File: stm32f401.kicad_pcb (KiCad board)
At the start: 2 copper layers, 35 x 35 mm, 37 parts, among them J1 USB_C_Receptacle_USB2.0_16P, SW1 SW_Push, SW2 SW_Push, U1 STM32F401RBT6, U2 BMI160, U3 AMS1117-3.3, Y1 16M

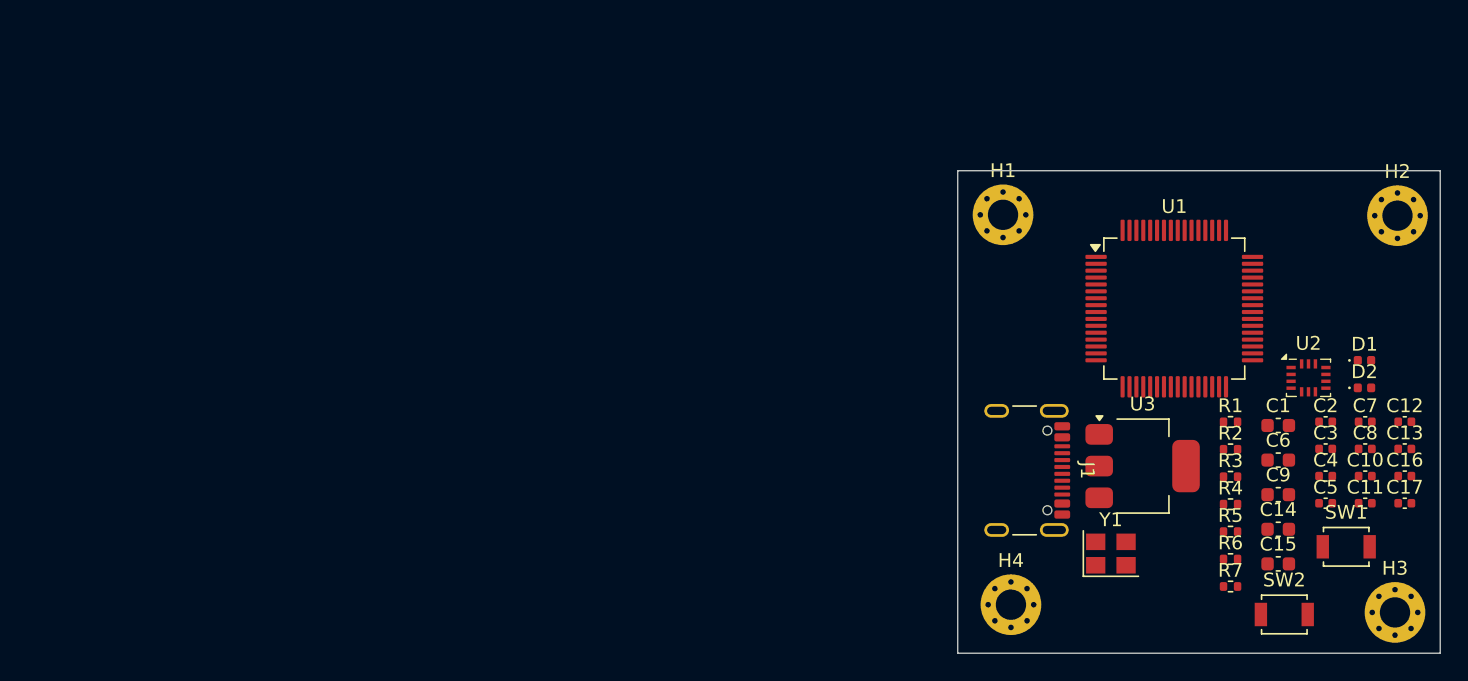
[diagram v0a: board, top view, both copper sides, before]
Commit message: Initial PCB Design
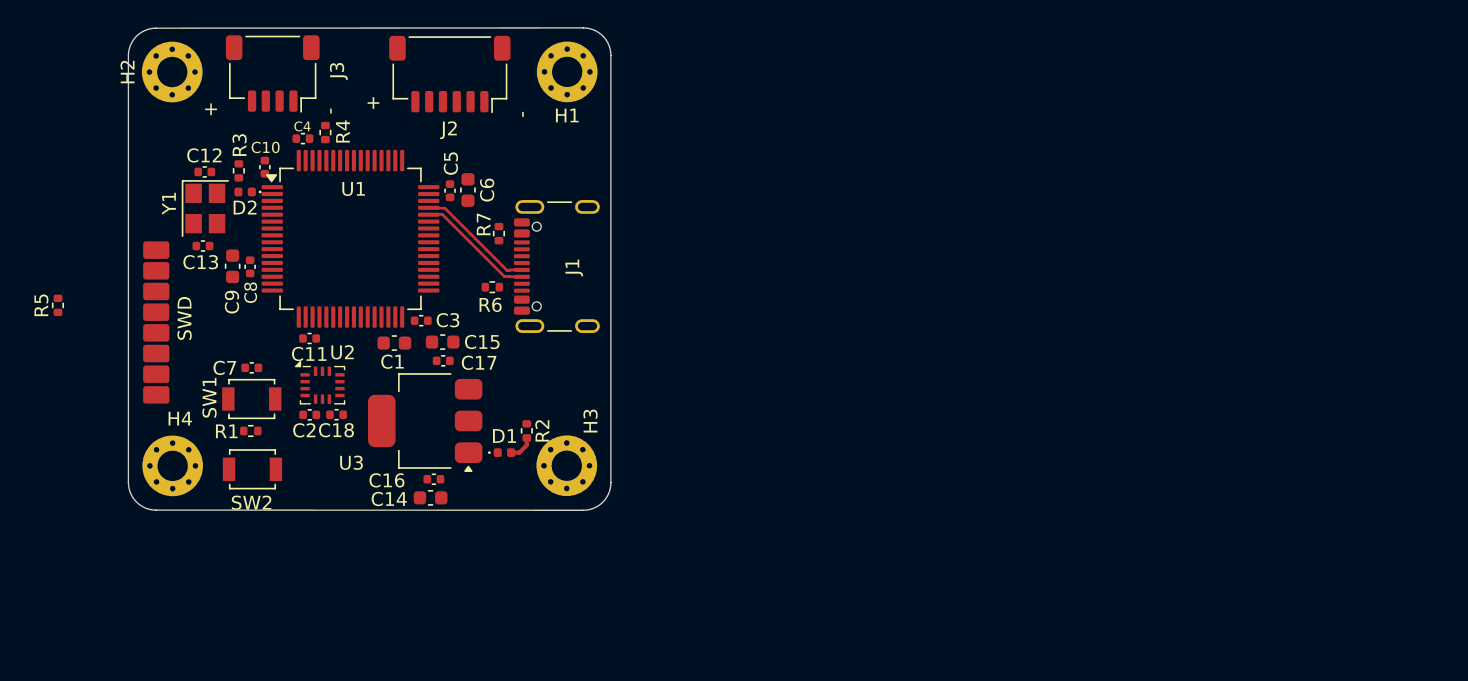
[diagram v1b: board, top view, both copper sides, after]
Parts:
- added C18: .1uF, Capacitor_SMD:C_0402_1005Metric, F.Cu at (55.1, 78.0)
- added J2: Conn_01x06_Pin, Connector_JST:JST_SH_SM06B-SRSS-TB_1x06-1MP_P1.00mm_Horizontal, F.Cu at (63.3, 53.3)
- added J3: Conn_01x04_Pin, Connector_JST:JST_SH_SM04B-SRSS-TB_1x04-1MP_P1.00mm_Horizontal, F.Cu at (50.5, 53.3)
- added SWD: Conn_01x08_Pin, Custom:Conn_0x08, F.Cu at (42.0, 80.6)
- D1: value RED -> R
- D2: value GREEN -> G
- moved H2 89.5 mm to (43.2, 53.2), turned to 90 degrees
- moved C12 88.9 mm to (45.5, 60.4)
- moved C13 88.4 mm to (45.4, 65.8)
- moved R5 86.6 mm to (34.9, 70.1), turned to 90 degrees
- moved C10 82.9 mm to (49.9, 60.1), turned to -90 degrees
- moved D2 82.4 mm to (48.5, 61.9), turned to 180 degrees
- moved C8 82.0 mm to (48.8, 67.3), turned to -90 degrees
- moved C7 80.9 mm to (49.0, 74.6)
- moved SW1 80.1 mm to (49.0, 76.9)
- moved C4 78.1 mm to (52.7, 58.0)
- moved C9 77.6 mm to (47.6, 67.3), turned to -90 degrees
- moved C11 77.5 mm to (53.1, 72.5), turned to 180 degrees
- moved SW2 75.6 mm to (49.0, 82.0)
- moved R3 75.3 mm to (48.0, 60.4), turned to -90 degrees
- moved C2 73.7 mm to (53.1, 78.0)
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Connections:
- net /NRST renamed NRST
- J1 pad S1: unconnected-(J1-SHIELD-PadS1) -> GND
- U1 pad 11: unconnected-(U1-PC3-Pad11) -> T3C4
- U1 pad 16: unconnected-(U1-PA2-Pad16) -> UART2_TX
- U1 pad 17: unconnected-(U1-PA3-Pad17) -> UART2_RX
- U1 pad 2: unconnected-(U1-PC13-Pad2) -> /USR_LED
- U1 pad 20: unconnected-(U1-PA4-Pad20) -> CS
- U1 pad 21: /USR_LED -> SCLK
- U1 pad 22: unconnected-(U1-PA6-Pad22) -> MISO
- U1 pad 23: unconnected-(U1-PA7-Pad23) -> MOSI
- U1 pad 24: unconnected-(U1-PC4-Pad24) -> T3C3
- U1 pad 25: unconnected-(U1-PC5-Pad25) -> T3C2
- U1 pad 37: unconnected-(U1-PC6-Pad37) -> T3C1
- U1 pad 46: unconnected-(U1-PA13-Pad46) -> SWDIO
- U1 pad 49: unconnected-(U1-PA14-Pad49) -> SWCLK
- U1 pad 55: unconnected-(U1-PB3-Pad55) -> SWO
- U1 pad 58: unconnected-(U1-PB6-Pad58) -> I2C1_SCL
- U1 pad 59: unconnected-(U1-PB7-Pad59) -> I2C1_SDA
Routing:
- net USB_D-: track 0.00 -> 8.65 mm
- net USB_D+: track 0.00 -> 8.65 mm
- net Net-(D1-A): track 0.00 -> 1.89 mm
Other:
- outline, holes or cut-outs redrawn
- board text added: "+"
- board text added: "-"
